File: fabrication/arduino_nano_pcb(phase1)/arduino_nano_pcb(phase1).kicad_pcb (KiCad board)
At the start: 2 copper layers, 69.2 x 58 mm, 7 parts, among them J1 Conn_02x04_Odd_Even, J2 Conn_01x04_Pin

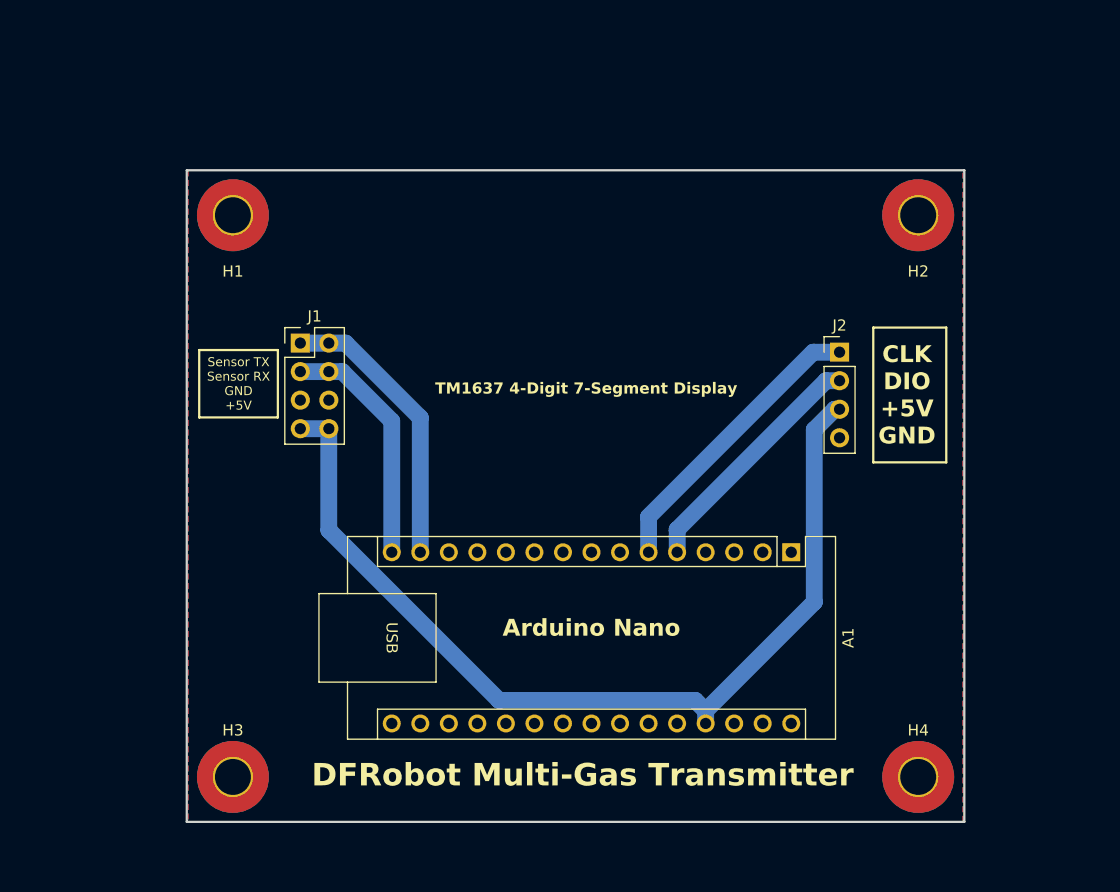
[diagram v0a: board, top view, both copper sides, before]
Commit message: feat(pcb_rev2): modified the pcb (rev 2)
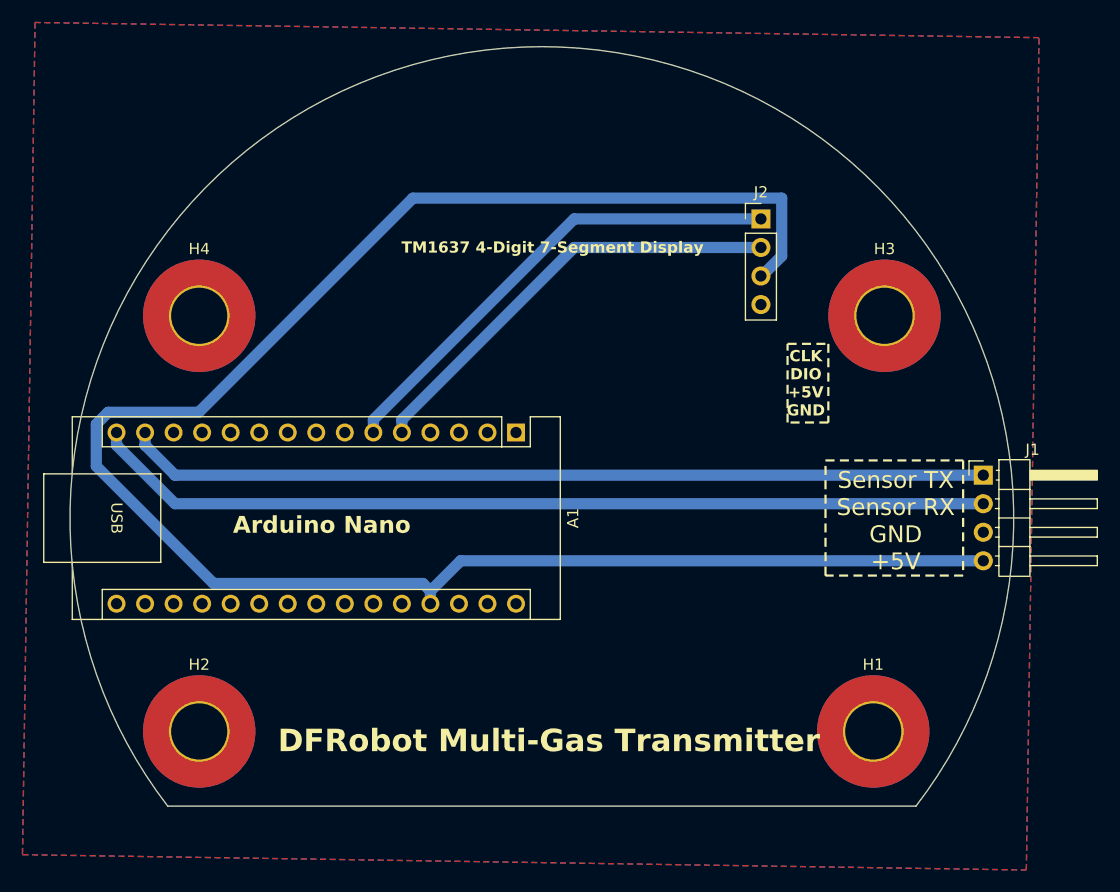
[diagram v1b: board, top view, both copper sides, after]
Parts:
- H1: renamed from H4; footprint MountingHole:MountingHole_3.2mm_M3_Pad_TopBottom -> MountingHole:MountingHole_5mm_Pad_TopBottom
- H2: renamed from H3; footprint MountingHole:MountingHole_3.2mm_M3_Pad_TopBottom -> MountingHole:MountingHole_5mm_Pad_TopBottom
- H3: renamed from H2; footprint MountingHole:MountingHole_3.2mm_M3_Pad_TopBottom -> MountingHole:MountingHole_5mm_Pad_TopBottom
- H4: renamed from H1; footprint MountingHole:MountingHole_3.2mm_M3_Pad_TopBottom -> MountingHole:MountingHole_5mm_Pad_TopBottom
- J1: value Conn_02x04_Odd_Even -> Conn_01x04_Pin; footprint Connector_PinHeader_2.54mm:PinHeader_2x04_P2.54mm_Vertical -> Connector_PinHeader_2.54mm:PinHeader_1x04_P2.54mm_Horizontal
- J2: footprint Connector_PinHeader_2.54mm:PinHeader_1x04_P2.54mm_Vertical -> TM1637:TM1637
- moved J1 61.9 mm to (114.3, 86.1)
- moved A1 26.7 mm to (72.7, 82.3)
- moved J2 13.8 mm to (94.5, 63.3)
- moved H3 9.44 mm to (105.5, 72.0)
- moved H4 9.44 mm to (44.5, 72.0)
- moved H1 5.69 mm to (104.5, 109.0)
- moved H2 5.04 mm to (44.5, 109.0)
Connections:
- J1 pad 2: /MCU_RX_SENSOR_TX -> /MCU_TX_SENSOR_RX
- J1 pad 3: /MCU_TX_SENSOR_RX -> GND
- J1 pad 4: /MCU_TX_SENSOR_RX -> VCC
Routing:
- net VCC: track 84.9 -> 166.6 mm
- net /MCU_TX_SENSOR_RX: track 21.6 -> 80.4 mm
- net /MCU_RX_SENSOR_TX: track 25.4 -> 76.9 mm
- net /TM1637_DIO: track 22.0 -> 39.4 mm
- net /TM1637_CLK: track 26.2 -> 43.0 mm
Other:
- board size 69.2 x 58 mm -> 84 x 67.6 mm
